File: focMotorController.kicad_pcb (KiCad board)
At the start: 4 copper layers, 73.3 x 56.5 mm, 55 parts, among them J2 JST-PH encoder connection, P1 WJ128V-5.0-3P, P2 Power input, U1 74LVC2T45DC, U10 IR2104 Gate Driver B, U11 IR2104 Gate Driver C, U12 Amplifier A, U13 Amplifier B, U14 Amplifier C, U2 74LVC2T45DC, U3 MOSFET A low, U4 MOSFET B low, U5 MOSFET C low, U6 MOSFET A high, U7 MOSFET B high, U8 MOSFET C high, U9 IR2104 Gate Driver A

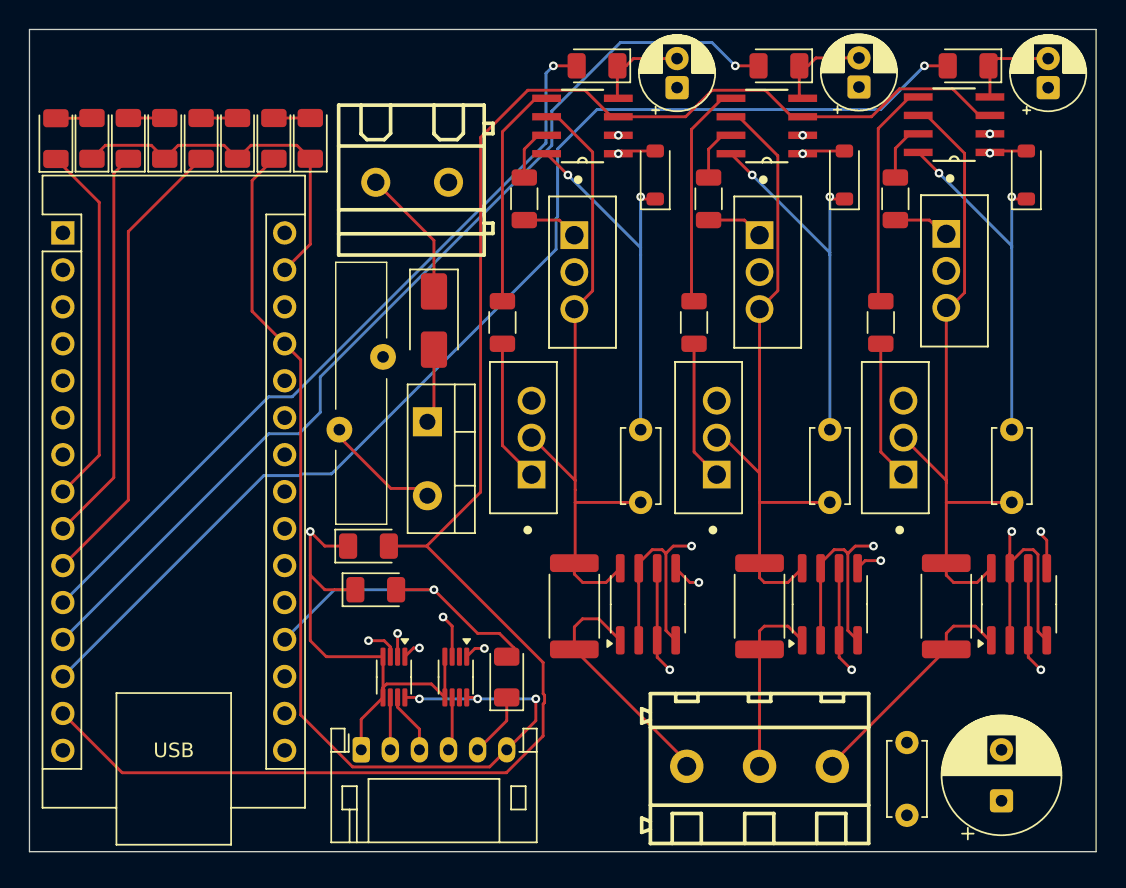
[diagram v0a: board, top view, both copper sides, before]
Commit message: Finish initial PCB version
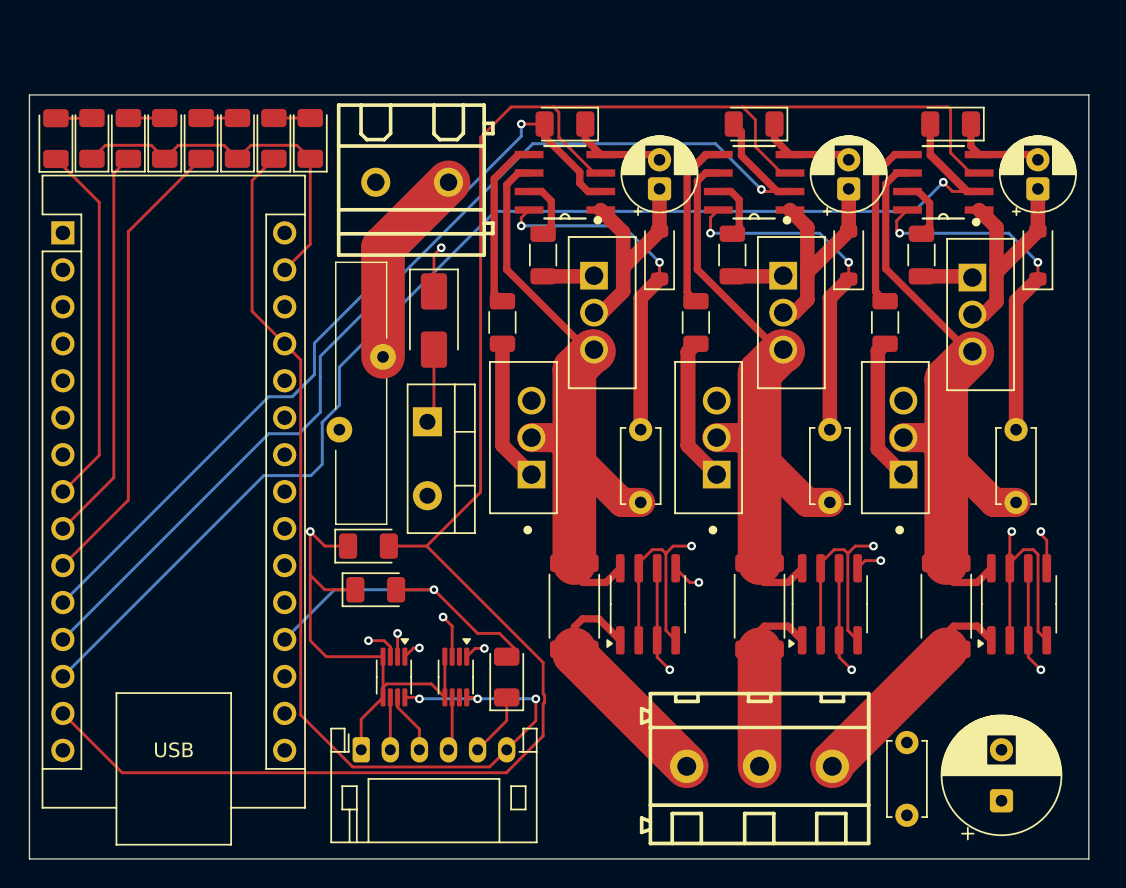
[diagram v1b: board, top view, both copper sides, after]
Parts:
- moved C8 7.06 mm to (116.5, 44.0)
- moved C6 7.04 mm to (129.5, 44.0)
- moved C7 6.99 mm to (142.5, 44.0)
- moved D9 5.56 mm to (142.5, 48.5)
- moved D7 5.51 mm to (116.5, 48.5)
- moved D8 5.51 mm to (129.5, 48.5)
- moved R7 4.57 mm to (110.0, 39.5)
- moved R8 4.35 mm to (123.0, 39.5)
- moved R12 4.26 mm to (134.5, 48.5)
- moved R9 4.19 mm to (121.5, 48.5)
- moved R11 4.18 mm to (136.5, 39.5)
- moved R22 4.08 mm to (108.5, 48.5)
- moved U9 4.05 mm to (110.0, 43.5)
- moved U11 4.03 mm to (136.0, 43.5)
- moved U10 3.96 mm to (123.0, 43.5)
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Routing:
- net PVIN: track 155.7 -> 107.2 mm, vias 3 -> 0
- net GND: track 344.8 -> 315.6 mm, vias 4 -> 5
- net Enable: track 124.1 -> 136.5 mm
- net CurrentC: track 55.1 -> 67.5 mm
- net BLowGate: track 9.64 -> 19.7 mm
- net Net-(U11-LO): track 14.8 -> 23.8 mm
- net Net-(U10-LO): track 14.9 -> 23.1 mm
- net Net-(D2-A): track 7.52 -> 0.00 mm
- net Net-(U9-LO): track 14.9 -> 22.4 mm
- net PhaseC: track 88.8 -> 94.0 mm, vias 2 -> 1
- net PhaseA: track 60.0 -> 55.2 mm, vias 2 -> 1
- net CurrentB: track 42.9 -> 47.1 mm
- net Net-(D8-K): track 27.2 -> 24.2 mm
- net Net-(D7-K): track 26.7 -> 23.9 mm
- net CLowGate: track 9.64 -> 12.1 mm
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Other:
- board size 73.3 x 56.5 mm -> 72.8 x 52.5 mm
